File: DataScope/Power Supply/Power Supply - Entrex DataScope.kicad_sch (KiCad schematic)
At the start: 128 parts, among them J2 Power Port, Q1 MPS3638, Q10 PN3569, Q11 PS3638, Q12 2N4918, Q13 2N3055, Q14 PN3569, Q15 PS3638, Q16 PN3569, Q17 PN3569, Q18 PS3638, Q19 JE520, Q2 PN3569, Q20 PN3569, Q3 PN3569, Q4 PS3638, Q5 2N4918, Q6 2N3055, Q7 PN3569, Q8 PS3638, Q9 PN3569

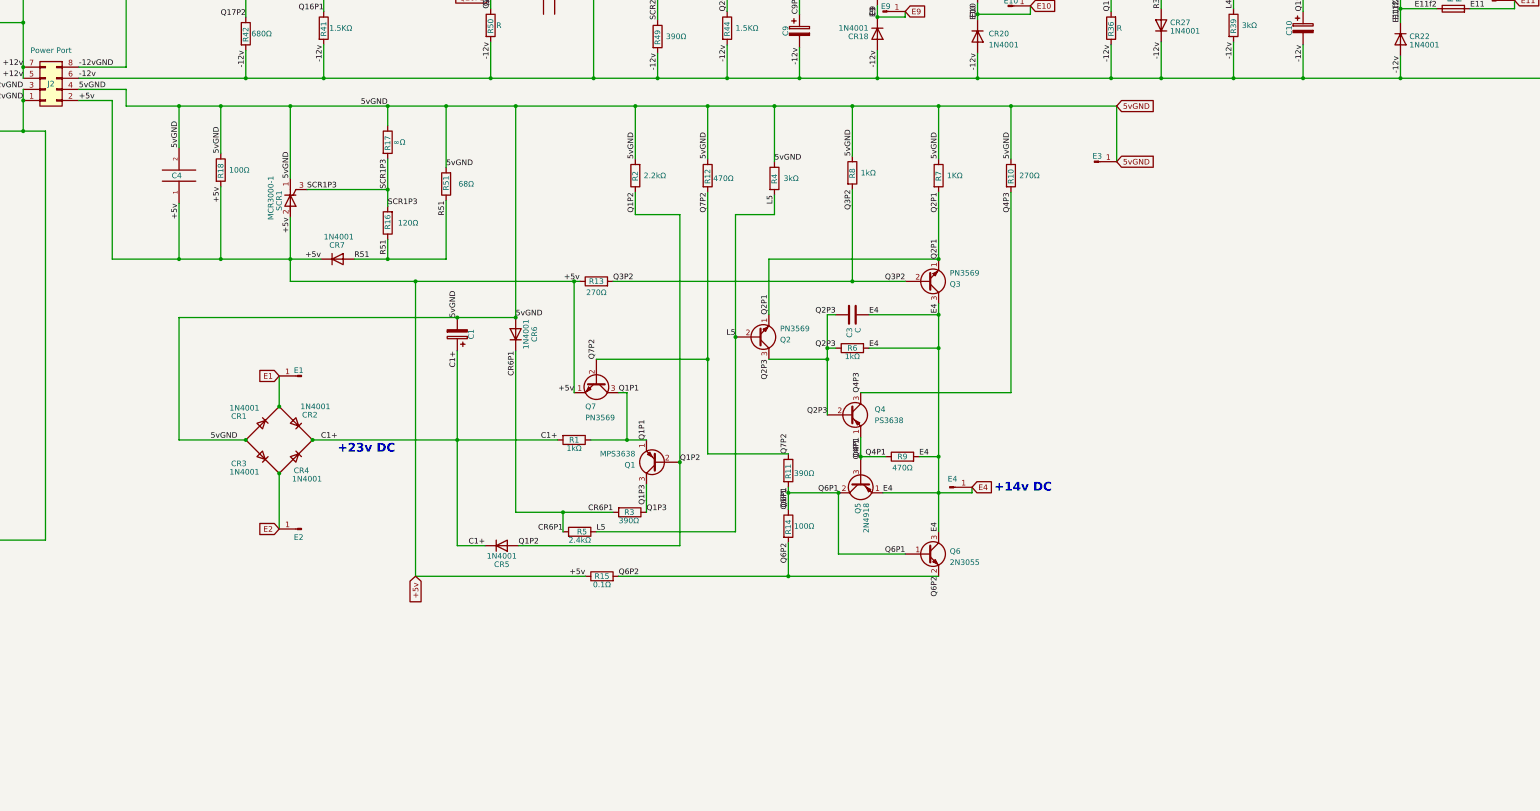
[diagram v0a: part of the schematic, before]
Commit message: mpre
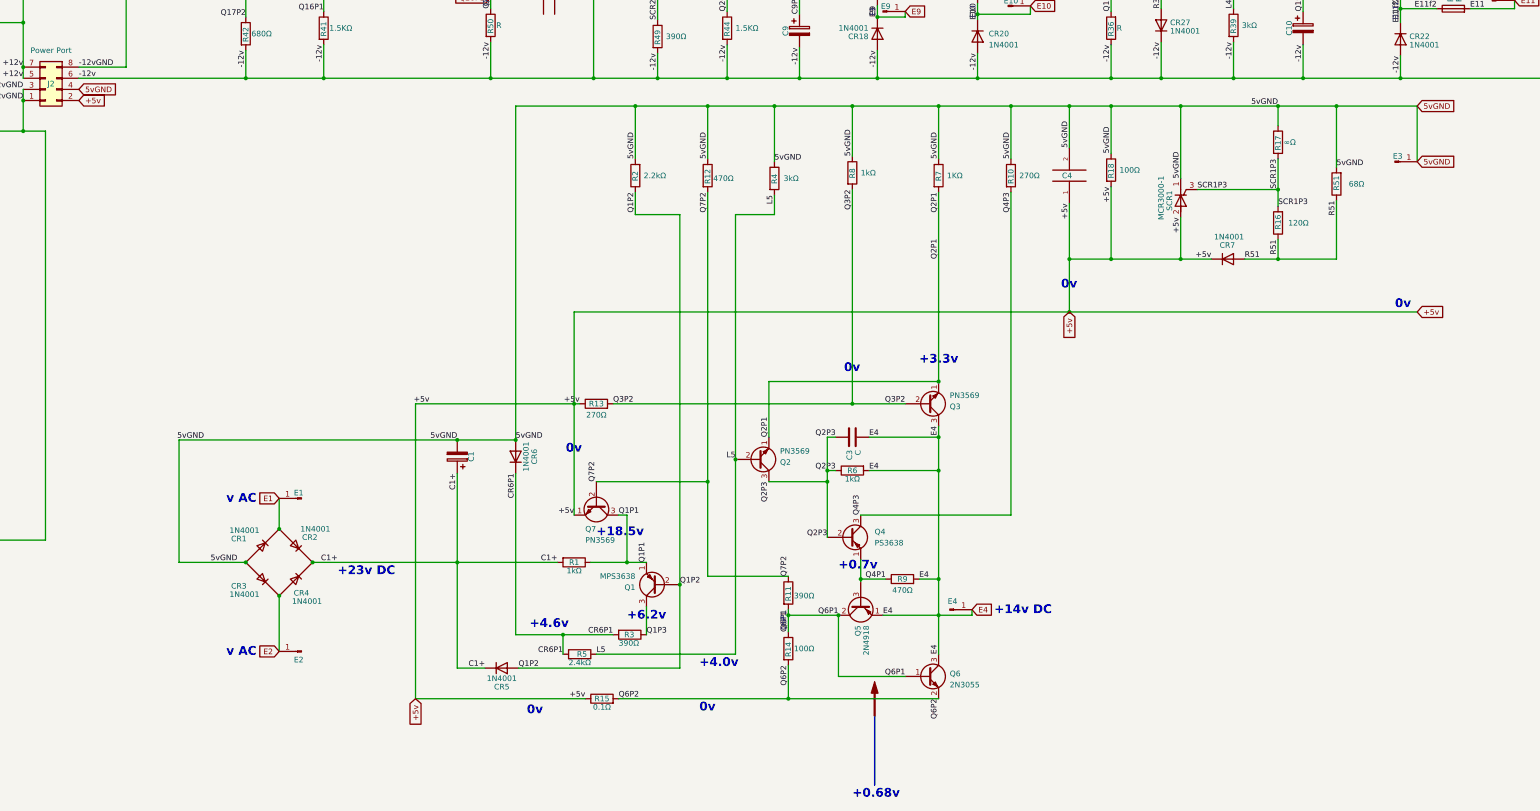
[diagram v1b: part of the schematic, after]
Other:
- note added: "+0.68v"
- note added: "+0.7v"
- note added: "+18.5v"
- note added: "+3.3v"
- note added: "+4.0v"
- note added: "+4.6v"
- note added: "+6.2v"
- note added: "0v"
- note added: "v AC"
- moved on the sheet: C1, C3, C4, CR1, CR2, CR3, CR4, CR5, CR6, CR7, E1, E2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
